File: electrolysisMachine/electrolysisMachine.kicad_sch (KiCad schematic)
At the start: 19 parts

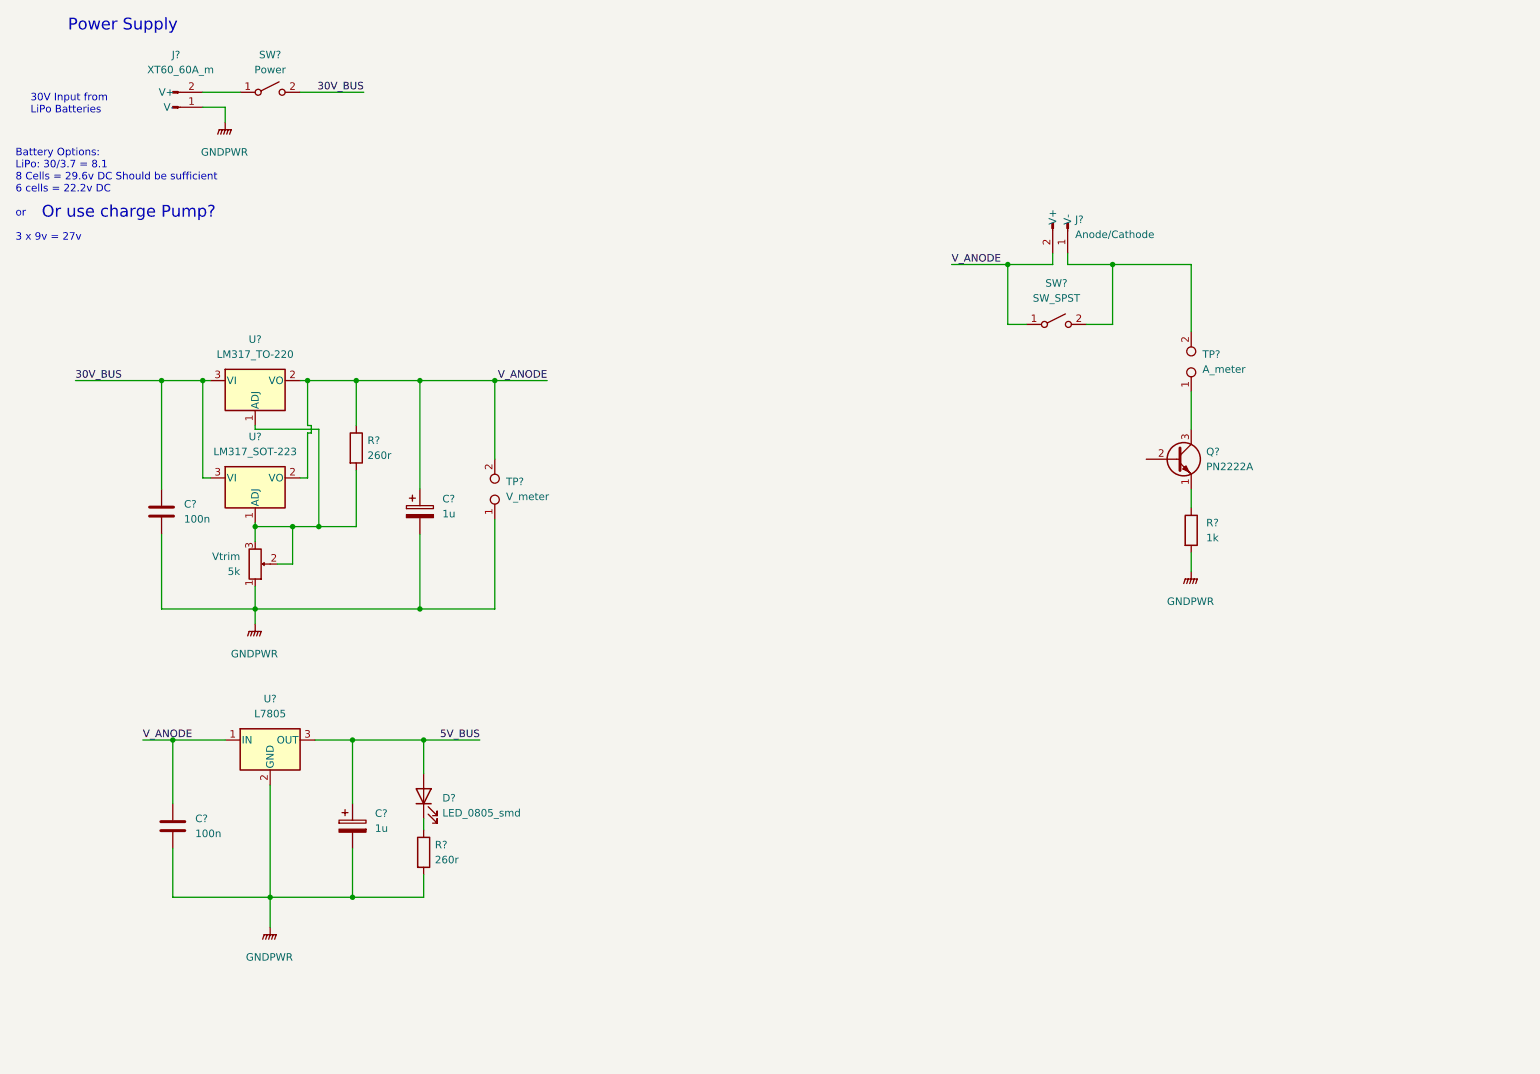
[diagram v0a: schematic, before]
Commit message: schem
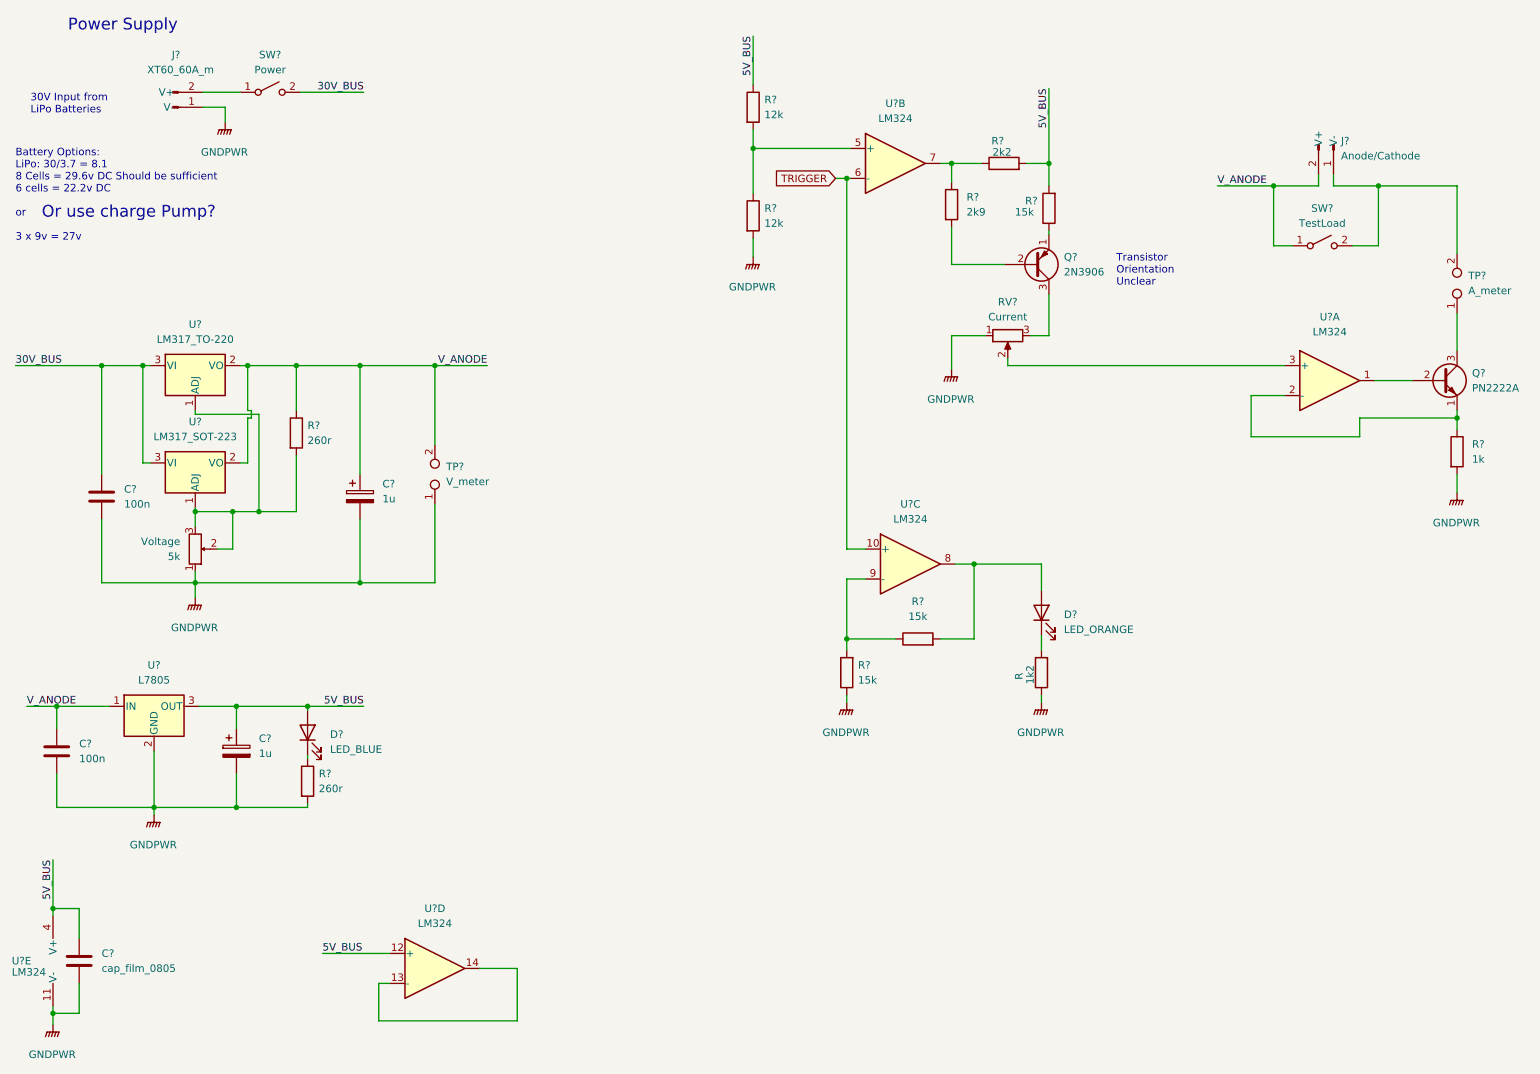
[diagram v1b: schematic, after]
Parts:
- added C?: cap_film_0805, Capacitor_SMD:C_0805_2012Metric_Pad1.18x1.45mm_HandSolder, symbol 000_Capacitor_FIlm_Immo:cap_film_0805
- added D?: LED_ORANGE, Diode_SMD:D_0805_2012Metric_Pad1.15x1.40mm_HandSolder, symbol 000_Diodes_Immo:LED_0805_smd
- added Q?: 2N3906, Package_TO_SOT_THT:TO-92_Inline, symbol Transistor_BJT:2N3906
- added R: 1k2, Resistor_SMD:R_0805_2012Metric_Pad1.20x1.40mm_HandSolder, symbol 000_Resistors_Immo:Resistor_0805
- added R? (x2): 12k, Resistor_SMD:R_0805_2012Metric_Pad1.20x1.40mm_HandSolder, symbol 000_Resistors_Immo:Resistor_0805
- added R?: 2k9, Resistor_SMD:R_0805_2012Metric_Pad1.20x1.40mm_HandSolder, symbol 000_Resistors_Immo:Resistor_0805
- added R? (x3): 15k, Resistor_SMD:R_0805_2012Metric_Pad1.20x1.40mm_HandSolder, symbol 000_Resistors_Immo:Resistor_0805
- added R?: 2k2, Resistor_SMD:R_0805_2012Metric_Pad1.20x1.40mm_HandSolder, symbol 000_Resistors_Immo:Resistor_0805
- added RV?: Current, Potentiometer_THT:Potentiometer_Alpha_RD901F-40-00D_Single_Vertical, symbol Device:R_Potentiometer
- added U? (x5): LM324, symbol Amplifier_Operational:LM324
- D?: value LED_0805_smd -> LED_BLUE
- SW?: value SW_SPST -> TestLoad
- renumbered Vtrim to Voltage
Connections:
- net 5V_BUS: now also C?.1, R?.1, R?.2, R?.2, U?.12 (+), U?.4 (V+)
- net GNDPWR: now also C?.2, R.1, R?.1, R?.2, RV?.1, U?.11 (V-)
- net at Q?.1 (E), R?.1: now also U?.2 (-)
- net at Q?.2 (B): now also U?.1
- new net: U?.13 (-), U?.14
- new net: RV?.2, U?.3 (+)
- new net: R?.1, R?.2, U?.5 (+)
- new net: D?.1 (K), R.2
- new net: R?.1, R?.1, U?.7
- new net: Q?.2 (B), R?.2
- new net: R?.1, R?.2, U?.9 (-)
- new net: D?.2 (A), R?.2, U?.8
- new net: Q?.1 (E), R?.1
- new net: Q?.3 (C), RV?.3
- new net TRIGGER: U?.10 (+), U?.6 (-)
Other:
- note added: "Transistor Orientation Unclear"
- moved on the sheet: C?, D?, J?, Q?, R?, SW?, TP?, U?, Voltage

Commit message: 6y7iy
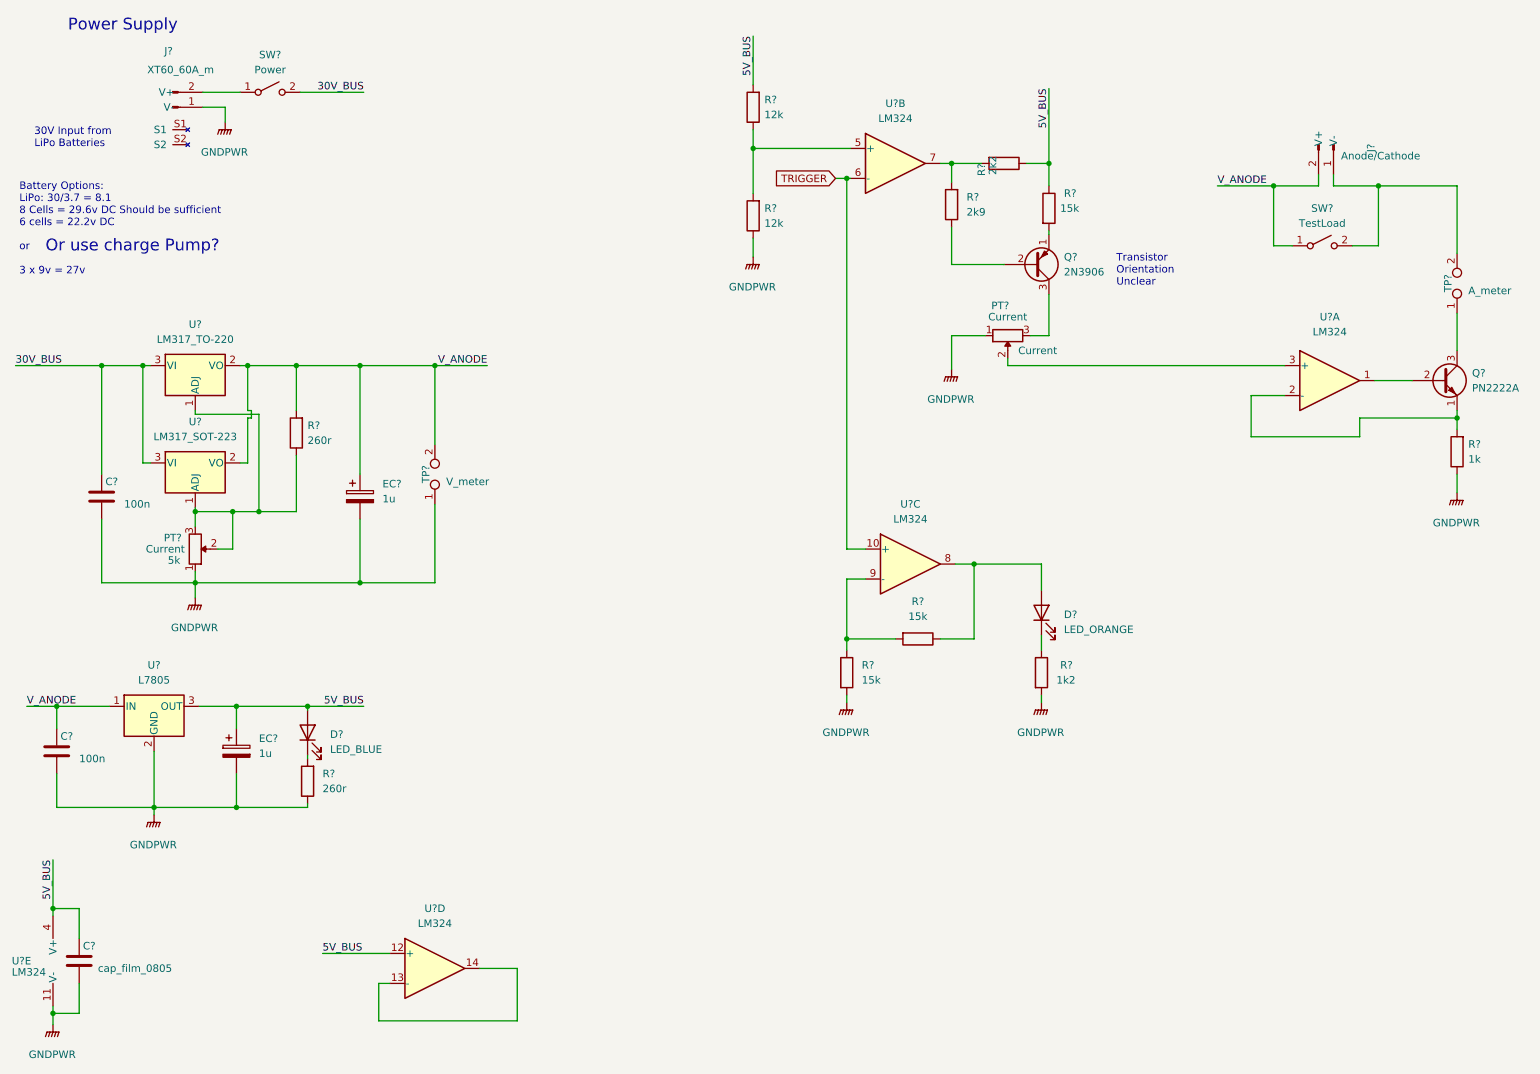
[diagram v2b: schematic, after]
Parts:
- removed C?: cap_film_0805, Capacitor_SMD:C_0805_2012Metric_Pad1.18x1.45mm_HandSolder, symbol 000_Capacitor_FIlm_Immo:cap_film_0805
- added C?: cap_film_0805, Capacitor_SMD:C_0805_2012Metric_Pad1.18x1.45mm_HandSolder, symbol 000_Capacitor_Film_Immo:cap_film_0805
- C? (x2): symbol 000_Capacitor_FIlm_Immo:cap_film_0805 -> 000_Capacitor_Film_Immo:cap_film_0805
- J?: symbol 000_Connectors_Immo:XT60_connector_DC_30A_female -> 000_Connectors_Immo:XT30_connector_DC_30A_female
- J?: symbol 000_Connectors_Immo:XT60_connector_DC_60A_male -> 000_Connectors_Immo:XT60_60A_male
- PT?: renamed from Voltage; footprint Potentiometer_THT:Potentiometer_Alps_RK09K_Single_Vertical -> Potentiometer_THT:Potentiometer_Alpha_RD901F-40-00D_Single_Vertical_CircularHoles; symbol Device:R_Potentiometer_Trim -> 000_Resistors_Immo:Potentiometer; Control (none) -> Current
- PT?: renamed from RV?; footprint Potentiometer_THT:Potentiometer_Alpha_RD901F-40-00D_Single_Vertical -> Potentiometer_THT:Potentiometer_Alpha_RD901F-40-00D_Single_Vertical_CircularHoles; symbol Device:R_Potentiometer -> 000_Resistors_Immo:Potentiometer; Control (none) -> Current
- Q?: footprint Package_TO_SOT_SMD:SOT-223-3_TabPin2 -> Package_TO_SOT_THT:TO-92_Inline
- U?: footprint Package_TO_SOT_THT:TO-220-3_Vertical -> Package_TO_SOT_SMD:SOT-223-3_TabPin2
- U?: footprint Package_SO:SOIC-8_3.9x4.9mm_P1.27mm -> Package_TO_SOT_THT:TO-220-3_Vertical
- gave numbers to parts that had none: 1
- renumbered R to R?
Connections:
- net 5V_BUS: now also R?.1, R?.1, R?.2, C?.1; no longer R?.1, R?.2, R?.2
- net GNDPWR: now also R?.1, R?.1, R?.1, R?.2, R?.2, C?.2; no longer R?.1, R?.1, R?.2, R?.2, R?.2
- net V_ANODE: now also R?.2; no longer R?.1
- net at PT?.2, PT?.3, U?.1 (ADJ)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: now also R?.1; no longer R?.2
- net at Q?.1 (E), U?.2 (-): now also R?.2; no longer R?.1
- net at D?.1 (K): now also R?.1; no longer R?.2
- net at Q?.2 (B): now also R?.1; no longer R?.2
- net at D?.1 (K): now also R?.2; no longer R?.1
- net at D?.2 (A), U?.8: now also R?.1; no longer R?.2
- net at Q?.1 (E): now also R?.2; no longer R?.1
- new net: R?.1, R?.2, U?.5 (+)
- new net: R?.2, R?.2, U?.7
- new net: R?.1, R?.2, U?.9 (-)
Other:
- moved on the sheet: R?
